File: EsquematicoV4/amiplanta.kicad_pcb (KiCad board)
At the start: 2 copper layers, 48 parts, among them J1 Jack-DC, J2 USB_B_Micro, J3 Conn_01x03_Female, Q1 SS8050-G, Q2 SS8050-G, U2 MAX98357AETE+, U3 ESP32-WROOM-32, U7 CP2102N-Axx-xQFN28

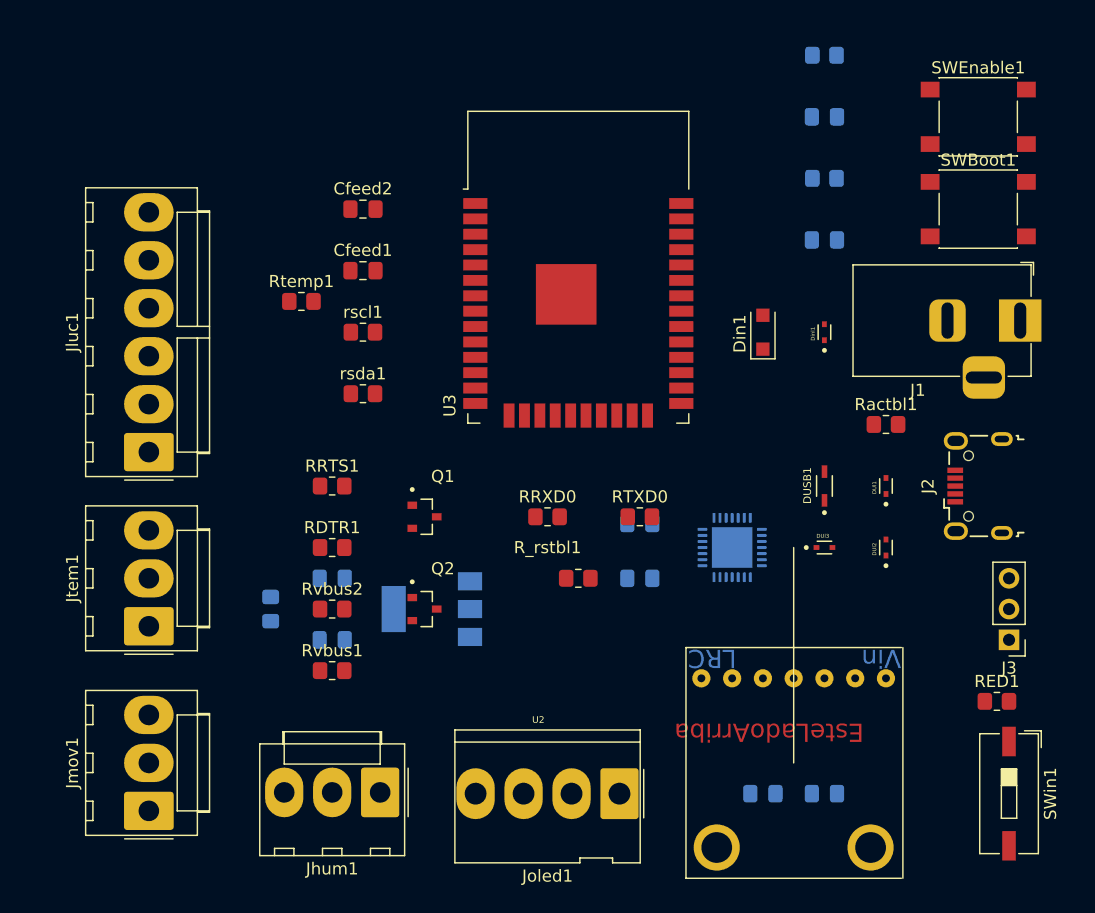
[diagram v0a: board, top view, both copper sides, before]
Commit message: PCB Final
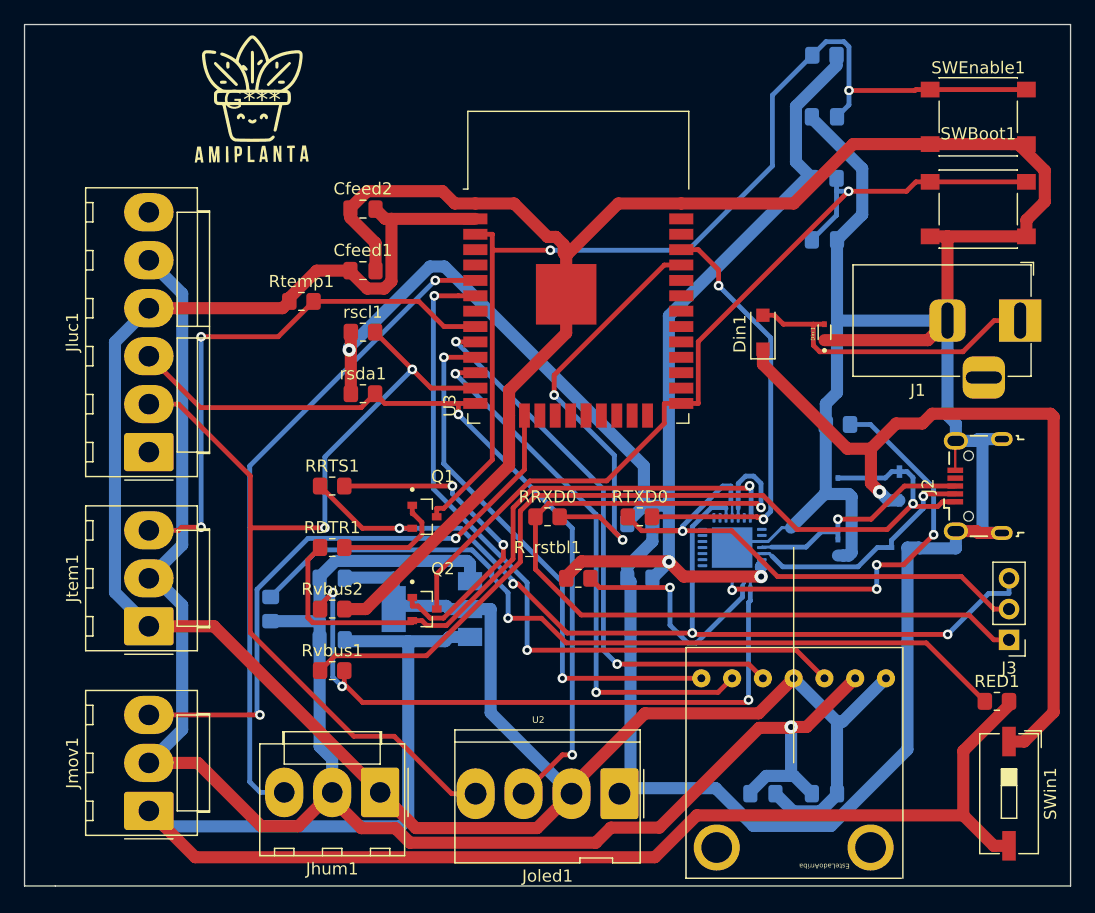
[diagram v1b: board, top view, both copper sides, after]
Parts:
- added G***: LOGO, AmplantaLogo:huellaAmiplantaLogo, F.Cu at (41.7, 46.9)
- DUSB1, DUl1, DUl2, DUl3, Ractbl1: moved to B.Cu
- moved DUSB1 6.19 mm to (95.1, 78.7)
- moved DUl3 6.19 mm to (95.1, 83.8), turned to 180 degrees
- moved DUl1 3.97 mm to (90.0, 78.7)
- moved DUl2 3.97 mm to (90.0, 83.8)
- moved Ractbl1 3.97 mm to (90.0, 73.7), turned to 180 degrees
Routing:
- net GNDREF: track 0.00 -> 305.6 mm
- net +3V3: track 0.00 -> 185.9 mm
- net GND: track 0.00 -> 162.6 mm, vias 0 -> 1
- net +5V: track 0.00 -> 133.4 mm
- net +3.3V: track 0.00 -> 116.3 mm, vias 0 -> 3
- net EN: track 0.00 -> 88.0 mm, vias 0 -> 2
- net /ESP32/SCL: track 0.00 -> 80.3 mm, vias 0 -> 2
- net /CP2102N-A02-GQFN28(Bootloader)/RTS: track 0.00 -> 78.9 mm, vias 0 -> 4
- net BOOT: track 0.00 -> 75.9 mm, vias 0 -> 1
- net /CP2102N-A02-GQFN28(Bootloader)/TXD: track 0.00 -> 72.3 mm, vias 0 -> 1
- net /CP2102N-A02-GQFN28(Bootloader)/VBUS: track 0.00 -> 72.0 mm, vias 0 -> 1
- net /ESP32/SDA: track 0.00 -> 67.8 mm, vias 0 -> 2
- net Net-(RED1-Pad1): track 0.00 -> 67.3 mm, vias 0 -> 1
- net +5V_Jack: track 0.00 -> 64.3 mm, vias 0 -> 1
- net /ESP32/amp_D_mode: track 0.00 -> 61.4 mm, vias 0 -> 2
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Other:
- board outline added: 86.4 x 71.1 mm
